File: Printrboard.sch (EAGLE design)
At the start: 131 parts, among them Q1 RFP30N06LE, Q2 RFP30N06LE, Q3 RFP30N06LE, Q4 RFP30N06LE, Q5 RFP30N06LE, U1 LM2841, U10 MCP4728, U2 A4982, U3 A4982, U4 A4982, U5 A4982, U6 AT90USB1286, U7 AP7313, U8 TXB0104, U9 PRTR5V0U4D, X1 16MHz

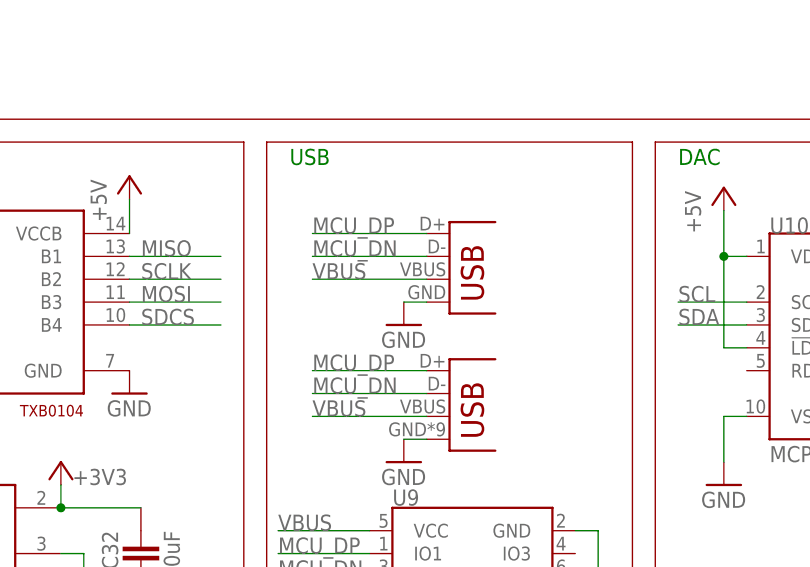
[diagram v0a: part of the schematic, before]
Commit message: Add in changes requested by PBHQ
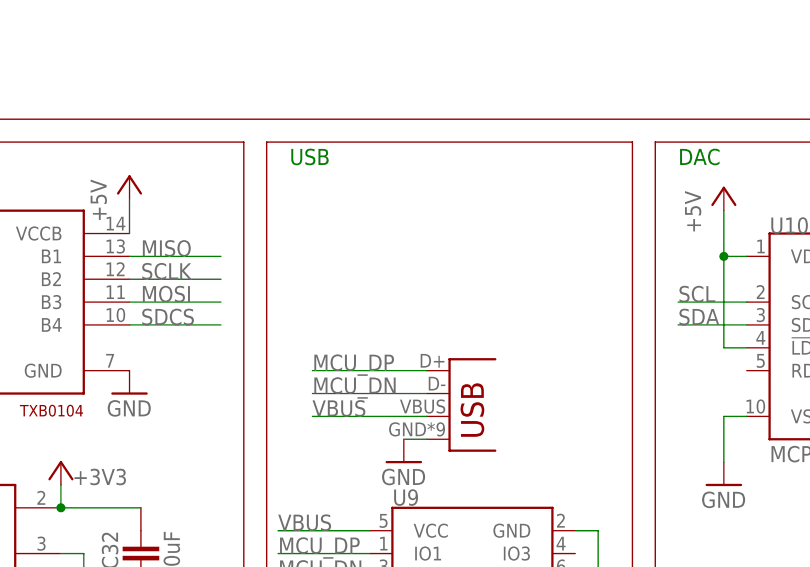
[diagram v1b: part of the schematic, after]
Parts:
- removed USB-B: USBPTH, printrbot:USBPTH
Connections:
- net GND: no longer USB-B.GND
- net MCU_DN: no longer USB-B.D-
- net MCU_DP: no longer USB-B.D+
- net VBUS: no longer USB-B.VBUS
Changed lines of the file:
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@@
 <part name="U9" library="printrbot" deviceset="PRTR5V0U4D" device=""/>
 <part name="GND53" library="SparkFun" deviceset="GND" device=""/>
-<part name="GND54" library="SparkFun" deviceset="GND" device=""/>
 <part name="U10" library="printrbot" deviceset="MCP4728" device=""/>
 <part name="GND56" library="SparkFun" deviceset="GND" device=""/>
@@
 <part name="Q4" library="ipc-7351-transistor" deviceset="MOSFET-NCH_" device="SOT-23" value="RFP30N06LE"/>
 <part name="U$6" library="12v" deviceset="12V" device=""/>
-<part name="USB-B" library="printrbot" deviceset="USB" device="PTH"/>
 <part name="SD" library="printrbot" deviceset="MICROSD-PP" device=""/>
 <part name="R23" library="ipc-7351-resistor" deviceset="RESISTOR_" device="0805" value="100k"/>
@@
 <instance part="U9" gate="G$1" x="119.38" y="-50.8"/>
 <instance part="GND53" gate="1" x="133.35" y="-59.69"/>
-<instance part="GND54" gate="1" x="111.76" y="-25.4"/>
 <instance part="U10" gate="G$1" x="165.1" y="-25.4"/>
 <instance part="GND56" gate="1" x="147.32" y="-43.18"/>
@@
 </instance>
 <instance part="U$6" gate="G$1" x="213.36" y="177.8"/>
-<instance part="USB-B" gate="G$1" x="116.84" y="-22.86"/>
 <instance part="SD" gate="G$1" x="12.7" y="-33.02"/>
 <instance part="R23" gate="G$1" x="71.12" y="213.36" rot="R270"/>
@@
 </segment>
 <segment>
-<wire x1="114.3" y1="-22.86" x2="111.76" y2="-22.86" width="0.1524" layer="91"/>
-<pinref part="GND54" gate="1" pin="GND"/>
-<pinref part="USB-B" gate="G$1" pin="GND"/>
-</segment>
-<segment>
 <pinref part="U10" gate="G$1" pin="VSS"/>
 <pinref part="GND56" gate="1" pin="GND"/>
@@
 </segment>
 <segment>
-<wire x1="114.3" y1="-17.78" x2="101.6" y2="-17.78" width="0.1524" layer="91"/>
-<label x="101.6" y="-17.78" size="1.778" layer="95"/>
-<pinref part="USB-B" gate="G$1" pin="D-"/>
-</segment>
-<segment>
 <pinref part="U9" gate="G$1" pin="IO2"/>
 <wire x1="107.95" y1="-53.34" x2="97.79" y2="-53.34" width="0.1524" layer="91"/>
@@
 <pinref part="R8" gate="G$1" pin="1"/>
 <label x="30.48" y="39.37" size="1.778" layer="95"/>
-</segment>
-<segment>
-<wire x1="114.3" y1="-15.24" x2="101.6" y2="-15.24" width="0.1524" layer="91"/>
-<label x="101.6" y="-15.24" size="1.778" layer="95"/>
-<pinref part="USB-B" gate="G$1" pin="D+"/>
 </segment>
 <segment>
@@
 </segment>
 <segment>
-<wire x1="114.3" y1="-20.32" x2="101.6" y2="-20.32" width="0.1524" layer="91"/>
-<label x="101.6" y="-20.32" size="1.778" layer="95"/>
-<pinref part="USB-B" gate="G$1" pin="VBUS"/>
-</segment>
-<segment>
